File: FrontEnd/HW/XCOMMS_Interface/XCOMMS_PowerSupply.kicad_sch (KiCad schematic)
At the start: 75 parts

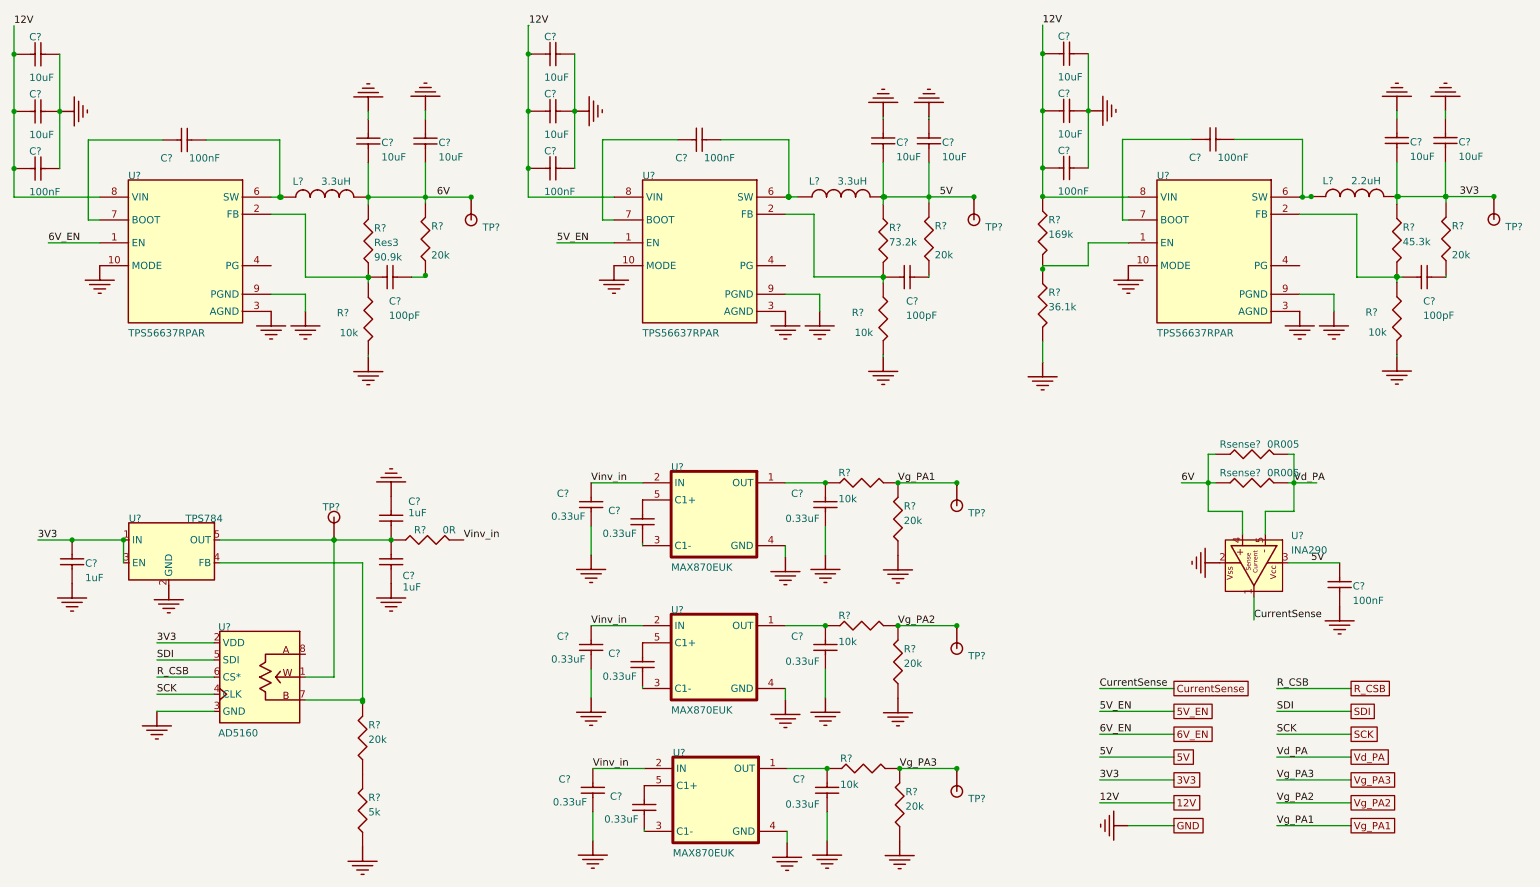
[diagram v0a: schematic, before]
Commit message: Altium to KiCad translation of interface board
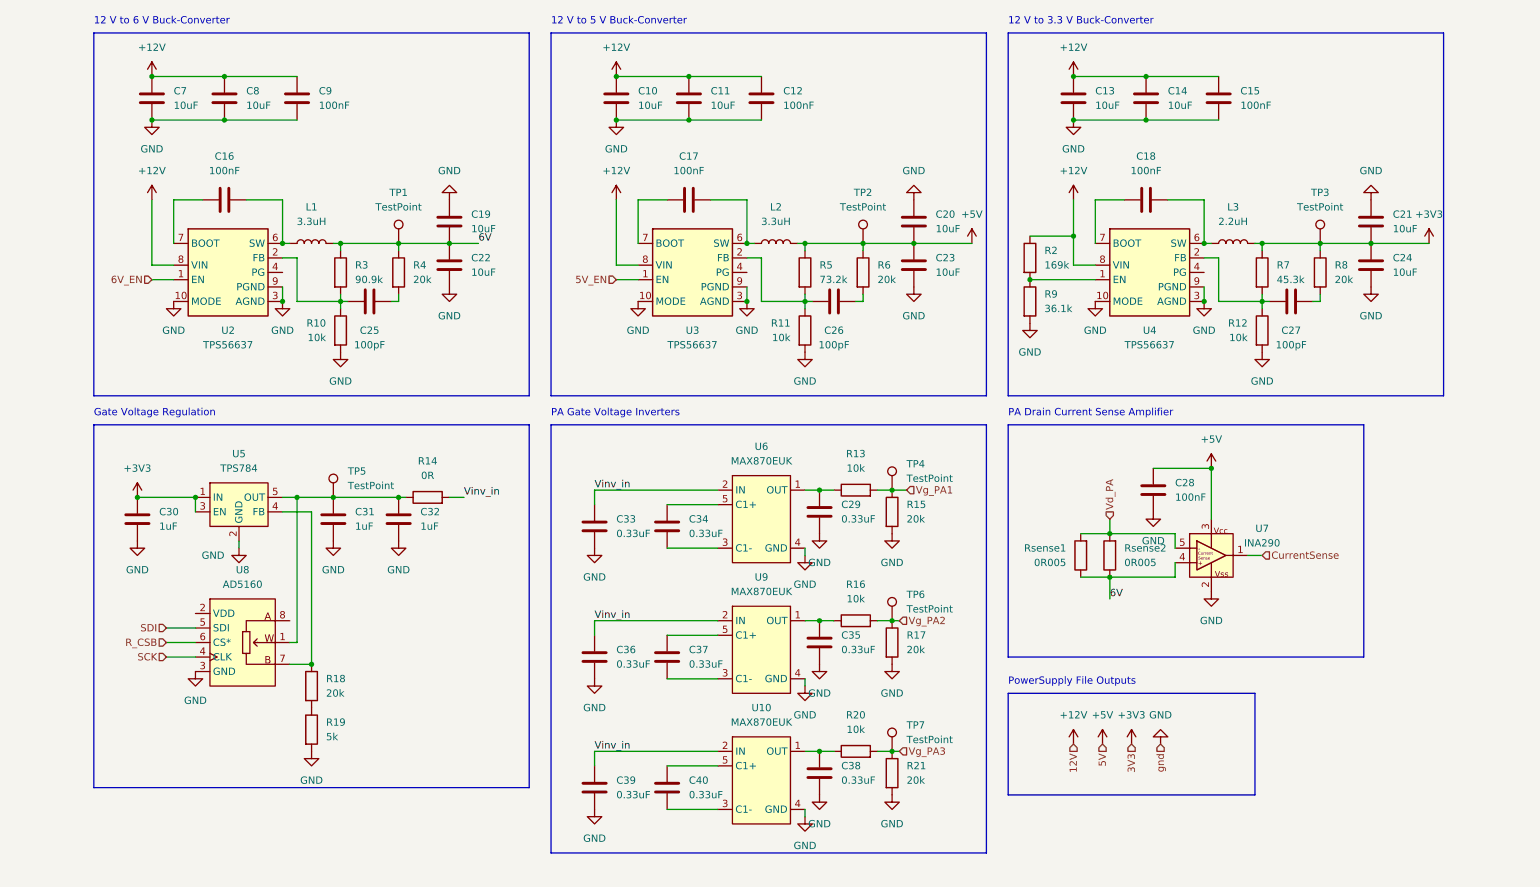
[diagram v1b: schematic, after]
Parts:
- removed C? (x3): Cap Semi, 0603 SMD Capacitor, symbol PowerSupply-altium-import:2_Cap Semi
- removed C? (x6): Cap Semi, 0805 SMD Capacitor, symbol PowerSupply-altium-import:3_mirrored_Cap Semi
- removed C? (x6): Cap Semi, 0805 SMD Capacitor, symbol PowerSupply-altium-import:0_mirrored_Cap Semi
- removed C? (x11): Cap Semi, 0603 SMD Capacitor, symbol PowerSupply-altium-import:3_mirrored_Cap Semi
- removed C? (x3): Cap Semi, 0603 SMD Capacitor, symbol PowerSupply-altium-import:0_mirrored_Cap Semi
- removed C? (x3): Cap Semi, 0603 SMD Capacitor, symbol PowerSupply-altium-import:2_mirrored_Cap Semi
- removed C?: Cap Semi, 0603 SMD Capacitor, symbol PowerSupply-altium-import:3_Cap Semi
- removed C?: Cap Semi, 0603 SMD Capacitor, symbol PowerSupply-altium-import:1_mirrored_Cap Semi
- removed L? (x2): 652-SRP5030T-3R3M, Bourns_SRP5030T-3R3M, symbol PowerSupply-altium-import:0_Inductor
- removed L?: WE_74438356022, Coilcraft_XAL60xx, symbol PowerSupply-altium-import:0_Inductor
- removed R? (x9): Res3, 0603 SMD Resistor, symbol PowerSupply-altium-import:1_Res3
- removed R? (x4): Res3, 0603 SMD Resistor, symbol PowerSupply-altium-import:0_Res3
- removed R? (x7): Res3, 0603 SMD Resistor, symbol PowerSupply-altium-import:3_Res3
- removed Rsense? (x2): Res3, 1206 SMD RESISTOR, symbol PowerSupply-altium-import:0_Res3
- removed TP? (x6): TP, TestPoint, symbol PowerSupply-altium-import:3_TP_d1.5mm
- removed TP?: TP, TestPoint, symbol PowerSupply-altium-import:1_TP_d1.5mm
- removed U? (x2): MAX870EUK, SOT23-5N, symbol PowerSupply-altium-import:0_MAX870EUK
- removed U? (x3): TPS56637RPAR, CONV_TPS56637RPAR, symbol PowerSupply-altium-import:0_TPS56637RPAR
- added C10, C11, C13, C14, C19, C20, C21, C22, C23, C24, C7, C8: 10uF, Capacitor_SMD:C_0805_2012Metric, symbol Device:C
- added C12, C15, C16, C17, C18, C28, C9: 100nF, Capacitor_SMD:C_0603_1608Metric, symbol Device:C
- added C25, C26, C27: 100pF, Capacitor_SMD:C_0603_1608Metric, symbol Device:C
- added C29, C33, C34, C35, C36, C37, C38, C39, C40: 0.33uF, Capacitor_SMD:C_0603_1608Metric, symbol Device:C
- added C30, C31, C32: 1uF, Capacitor_SMD:C_0603_1608Metric, symbol Device:C
- added L1, L2: 3.3uH, Inductor_SMD:L_Bourns_SRP5030T, symbol Device:L
- added L3: 2.2uH, Inductor_SMD:L_Coilcraft_XAL60xx_6.36x6.56mm, symbol Device:L
- added R10, R11, R12, R13, R16, R20: 10k, Resistor_SMD:R_0603_1608Metric, symbol Device:R
- added R14: 0R, Resistor_SMD:R_0603_1608Metric, symbol Device:R
- added R15, R17, R18, R21, R4, R6, R8: 20k, Resistor_SMD:R_0603_1608Metric, symbol Device:R
- added R19: 5k, Resistor_SMD:R_0603_1608Metric, symbol Device:R
- added R2: 169k, Resistor_SMD:R_0603_1608Metric, symbol Device:R
- added R3: 90.9k, Resistor_SMD:R_0603_1608Metric, symbol Device:R
- added R5: 73.2k, Resistor_SMD:R_0603_1608Metric, symbol Device:R
- added R7: 45.3k, Resistor_SMD:R_0603_1608Metric, symbol Device:R
- added R9: 36.1k, Resistor_SMD:R_0603_1608Metric, symbol Device:R
- added Rsense1, Rsense2: 0R005, Resistor_SMD:R_1206_3216Metric, symbol Device:R
- added TP1, TP2, TP3, TP4, TP5, TP6, TP7: TestPoint, TestPoint:TestPoint_Pad_D1.0mm, symbol Connector:TestPoint
- added U10, U9: MAX870EUK, Package_TO_SOT_SMD:SOT-23-5, symbol GGS_Power:MAX870
- added U2, U3, U4: TPS56637, GGS_Power:TPS56637RPAR, symbol GGS_Power:TPS56637
- U5: renamed from U?; footprint SOT23-5N -> Package_TO_SOT_SMD:SOT-23-5; symbol PowerSupply-altium-import:0_TPS784 -> GGS_Power:TPS784
- U6: renamed from U?; footprint SOT23-5N -> Package_TO_SOT_SMD:SOT-23-5; symbol PowerSupply-altium-import:0_MAX870EUK -> GGS_Power:MAX870
- U7: renamed from U?; footprint SC70-5 -> GGS_Miscellaneous:SC70-5; symbol PowerSupply-altium-import:3_INA290 -> GGS_Miscellaneous:INA290
- U8: renamed from U?; footprint SOT-28-8N -> Package_TO_SOT_SMD:SOT-23-8; symbol PowerSupply-altium-import:0_AD5160 -> GGS_Miscellaneous:AD1560
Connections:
- net 5V_EN: now also U3.1 (EN)
- net 6V: now also C19.1, C22.1, L1.2, R3.1, R4.1, Rsense1.1, Rsense2.1, TP1.1
- net 6V_EN: now also U2.1 (EN)
- net GND: now also C10.2, C11.2, C12.2, C13.2, C14.2, C15.2, C19.2, C20.2, C21.2, C22.2, C23.2, C24.2, C28.1, C29.1, C30.2, C31.2, C32.2, C33.1, C35.1, C36.1, C38.1, C39.1, C7.2, C8.2, C9.2, R10.2, R11.2, R12.2, R15.2, R17.2, R19.2, R21.2, R9.2, U10.4 (GND), U2.10 (MODE), U2.3 (AGND), U2.9 (PGND), U3.10 (MODE), U3.3 (AGND), U3.9 (PGND), U4.10 (MODE), U4.3 (AGND), U4.9 (PGND), U9.4 (GND)
- net Vd_PA: now also Rsense1.2, Rsense2.2
- net Vg_PA1: now also R13.2, R15.1, TP4.1
- net Vg_PA2: now also R16.2, R17.1, TP6.1
- net Vg_PA3: now also R20.2, R21.1, TP7.1
- net Vinv_in: now also C33.2, C36.2, C39.2, R14.2, U10.2 (IN), U9.2 (IN)
- net at U5.4 (FB), U8.7 (B): now also R18.1
- net at U5.5 (OUT), U8.1 (W): now also C31.1, C32.1, R14.1, TP5.1
- net at U6.1 (OUT): now also C29.2, R13.1
- net at U6.5 (C1+): now also C34.2
- net at U6.3 (C1-): now also C34.1
- net 3V3 renamed +3V3
- net +3V3: now also C21.1, C24.1, C30.1, L3.2, R7.1, R8.1, TP3.1; no longer U8.2 (VDD)
- net 5V renamed +5V
- net +5V: now also C20.1, C23.1, C28.2, L2.2, R5.1, R6.1, TP2.1
- new net: C17.1, U3.7 (BOOT)
- new net: C17.2, L2.1, U3.6 (SW)
- new net: C27.2, R8.2
- new net: C26.1, R11.1, R5.2, U3.2 (FB)
- new net: C18.1, U4.7 (BOOT)
- new net: C18.2, L3.1, U4.6 (SW)
- new net: R18.2, R19.1
- new net: C38.2, R20.1, U10.1 (OUT)
- new net: C16.1, U2.7 (BOOT)
- new net: C16.2, L1.1, U2.6 (SW)
- new net: C27.1, R12.1, R7.2, U4.2 (FB)
- new net: R2.2, R9.1, U4.1 (EN)
- new net: C25.1, R10.1, R3.2, U2.2 (FB)
- new net: C40.1, U10.3 (C1-)
- new net: C40.2, U10.5 (C1+)
- new net: C25.2, R4.2
- new net: C35.2, R16.1, U9.1 (OUT)
- new net: C26.2, R6.2
- new net: C37.1, U9.3 (C1-)
- new net: C37.2, U9.5 (C1+)
- new net +12V: C10.1, C11.1, C12.1, C13.1, C14.1, C15.1, C7.1, C8.1, C9.1, R2.1, U2.8 (VIN), U3.8 (VIN), U4.8 (VIN)
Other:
- note added: "12 V to 3.3 V Buck-Converter"
- note added: "12 V to 5 V Buck-Converter"
- note added: "12 V to 6 V Buck-Converter"
- note added: "Gate Voltage Regulation"
- note added: "PA Drain Current Sense Amplifier"
- note added: "PA Gate Voltage Inverters"
- note added: "PowerSupply File Outputs"
- moved on the sheet: U5, U6
